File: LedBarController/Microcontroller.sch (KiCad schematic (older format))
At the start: 29 parts, among them J1001 Conn_01x03, J1002 Conn_01x03, J1003 Conn_01x03, J1004 Conn_01x03, J1005 AVR-ISP-6, J1006 Conn_01x06, SW1001 SW_Push, U1001 ATmega328P-AU, Y1001 Crystal

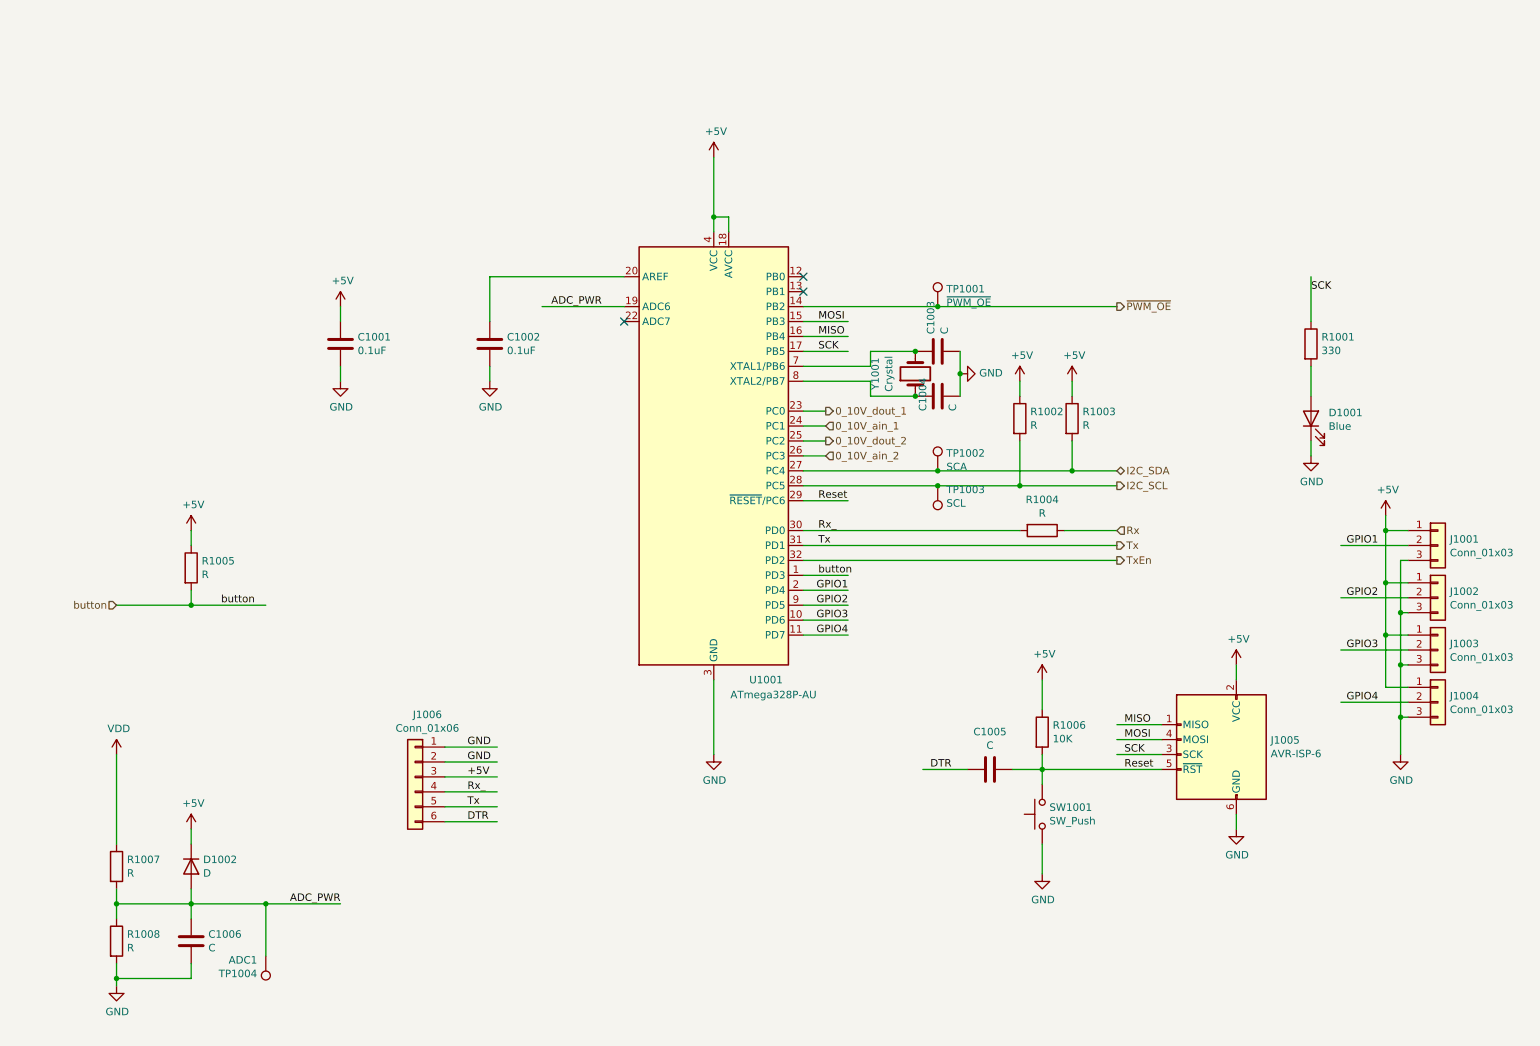
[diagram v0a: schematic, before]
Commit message: Updated schematic, added ds1307, replaced gpio-headers for LEDs and solder-jumpers and remove ISP-connector
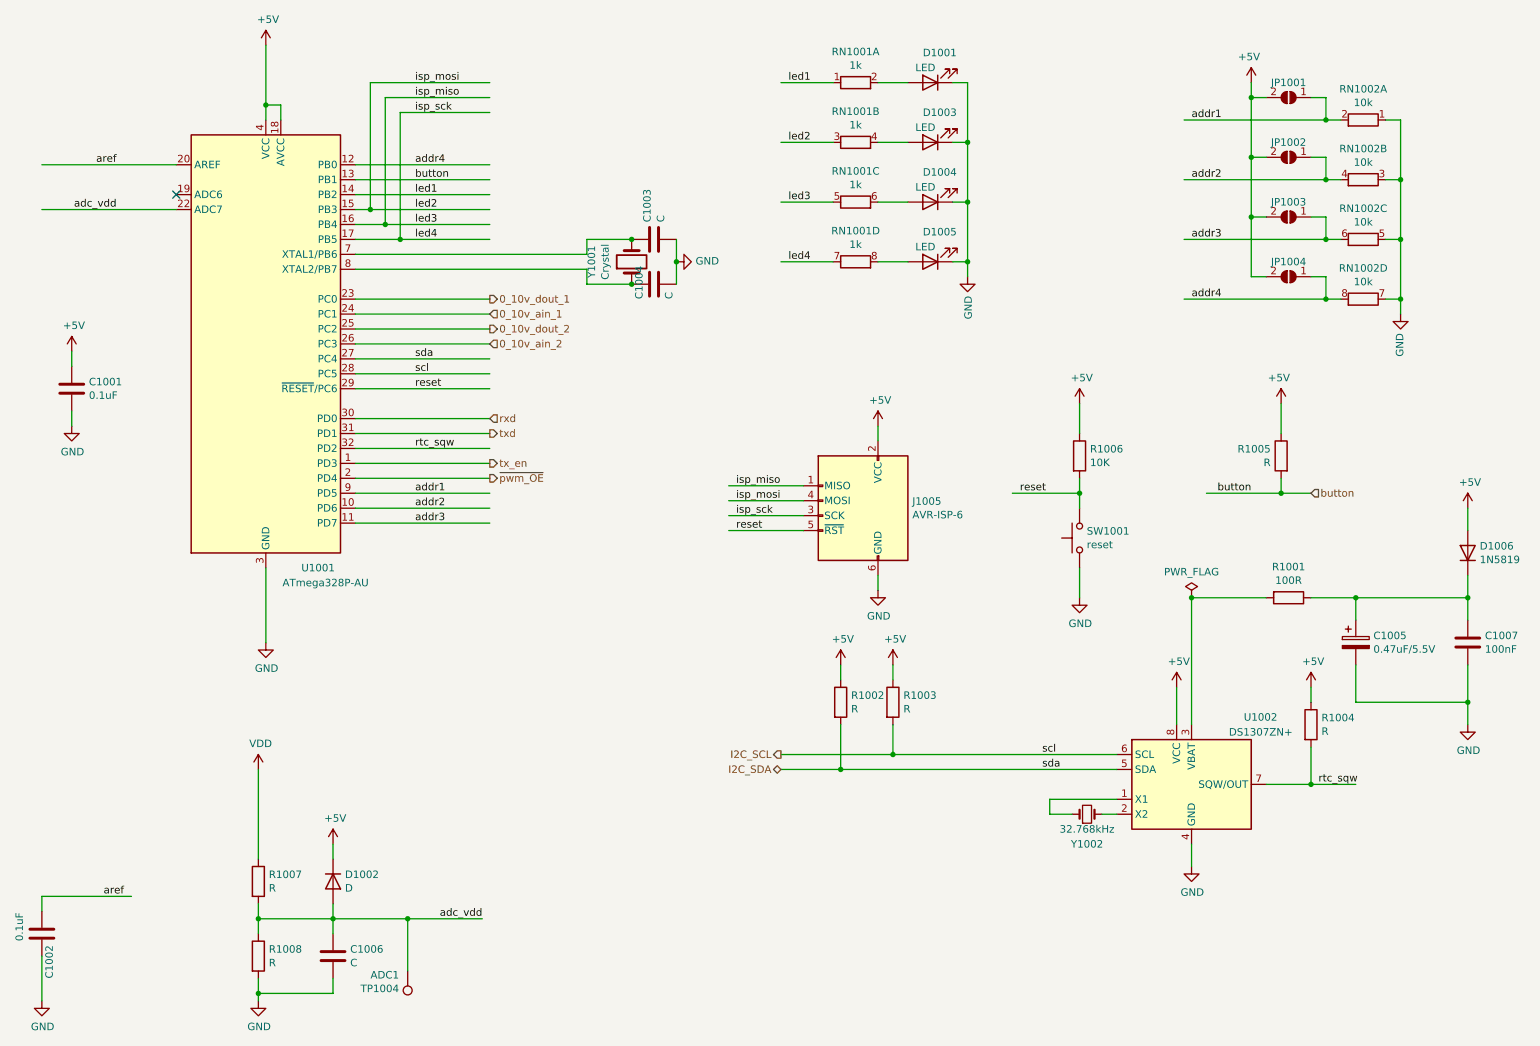
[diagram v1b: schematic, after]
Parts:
- removed C1005: C, Capacitor_SMD:C_0805_2012Metric_Pad1.18x1.45mm_HandSolder, symbol Device:C
- removed J1001, J1002, J1003, J1004: Conn_01x03, Connector_PinSocket_2.54mm:PinSocket_1x03_P2.54mm_Vertical, symbol Connector_Generic:Conn_01x03
- removed J1006: Conn_01x06, Connector_PinHeader_2.54mm:PinHeader_1x06_P2.54mm_Vertical, symbol Connector_Generic:Conn_01x06
- removed TP1001: ~PWM_OE, TestPoint:TestPoint_Pad_D1.0mm, symbol Connector:TestPoint
- removed TP1002: SCA, TestPoint:TestPoint_Pad_D1.0mm, symbol Connector:TestPoint
- removed TP1003: SCL, TestPoint:TestPoint_Pad_D1.0mm, symbol Connector:TestPoint
- added C1005: 0.47uF/5.5V, symbol Device:CP
- added C1007: 100nF, Capacitor_SMD:C_0805_2012Metric_Pad1.18x1.45mm_HandSolder, symbol Device:C
- added D1003, D1004, D1005: LED, LED_SMD:LED_0805_2012Metric_Pad1.15x1.40mm_HandSolder, symbol Device:LED
- added D1006: 1N5819, Diode_SMD:D_SOD-123, symbol Device:D
- added JP1001, JP1002, JP1003, JP1004: SolderJumper_2_Open, Jumper:SolderJumper-2_P1.3mm_Open_TrianglePad1.0x1.5mm, symbol Jumper:SolderJumper_2_Open
- added RN1001: 1k, Resistor_SMD:R_Array_Concave_4x0603, symbol Device:R_Pack04_SIP_Split
- added RN1002: 10k, Resistor_SMD:R_Array_Concave_4x0603, symbol Device:R_Pack04_SIP_Split
- added U1002: DS1307ZN+, Package_SO:SOIC-8_3.9x4.9mm_P1.27mm, symbol Timer_RTC:DS1307ZN+
- added Y1002: 32.768kHz, Crystal:Crystal_DS26_D2.0mm_L6.0mm_Vertical, symbol Device:Crystal_Small
- D1001: value Blue -> LED
- R1001: value 330 -> 100R
- SW1001: value SW_Push -> reset
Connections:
- net labels added: 0_10v_ain_1, 0_10v_ain_2, 0_10v_dout_1, 0_10v_dout_2, adc_vdd, addr1, addr2, addr3, addr4, aref, isp_miso, isp_mosi, isp_sck, led1, led2, led3, led4, reset, rtc_sqw, rxd, scl, sda, tx_en, txd, ~pwm_OE
- net labels removed: 0_10V_ain_1, 0_10V_ain_2, 0_10V_dout_1, 0_10V_dout_2, ADC_PWR, DTR, GPIO1, GPIO2, GPIO3, GPIO4, MISO, MOSI, Reset, Rx, Rx_, SCK, Tx, TxEn, ~PWM_OE
- wire segments 107 -> 157
- no-connect marks 3 -> 1
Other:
- moved on the sheet: C1001, C1002, C1003, C1004, C1006, D1002, J1005, R1002, R1003, R1005, R1006, R1007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
